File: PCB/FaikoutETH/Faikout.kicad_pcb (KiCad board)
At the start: 2 copper layers, 70 x 70 mm, 70 parts, among them J1 1x5, J2 TC2030-USB-NL, J3 Reset, J4 RJ45_LED, Q1 BSS138PS, U1 KSZ8851SNL, U4 ESP32-S3-MINI-1, U5 TPS62933, Y1 Crystal_GND24

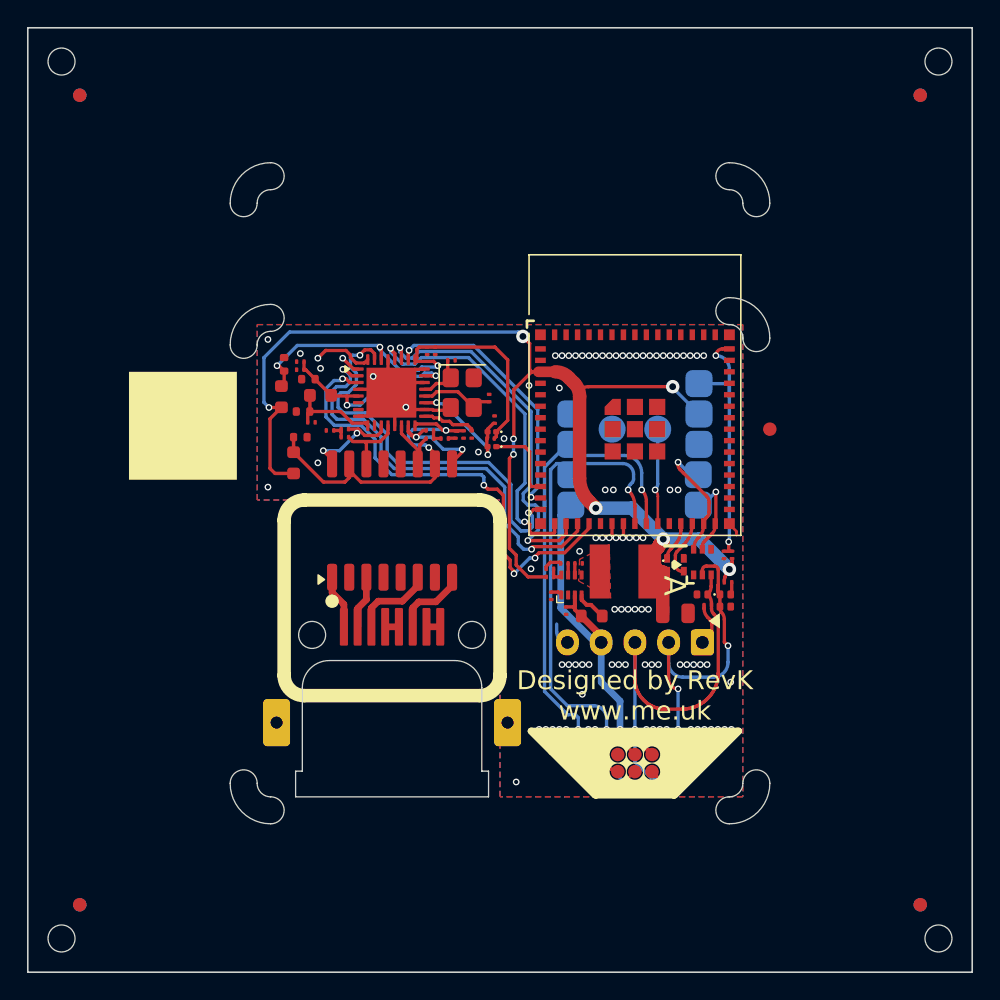
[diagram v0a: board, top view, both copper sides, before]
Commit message: Rotate
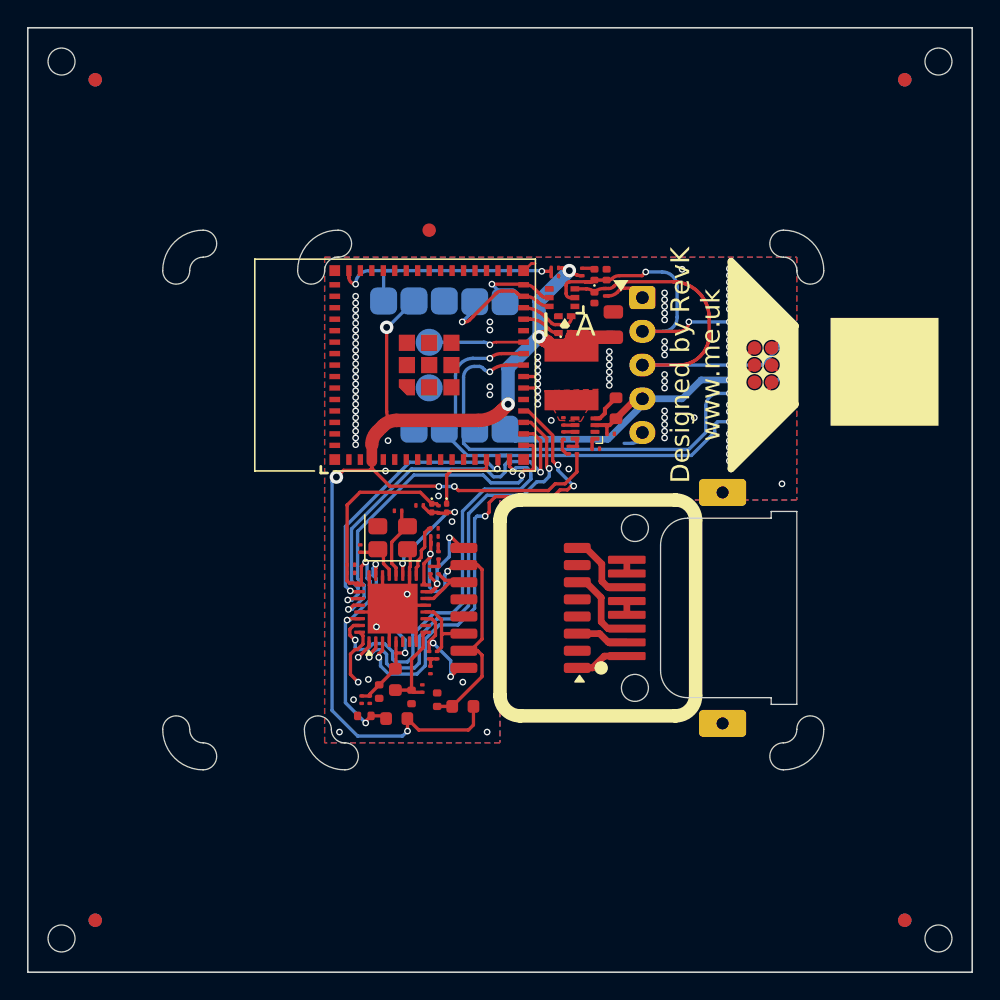
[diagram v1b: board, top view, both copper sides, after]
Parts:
- moved V5 32.5 mm to (112.0, 65.0), turned to 90 degrees
- moved V6 31.1 mm to (157.0, 65.0), turned to 90 degrees
- moved J2 31.0 mm to (154.5, 55.0), turned to -90 degrees
- moved FID2 29.2 mm to (129.8, 45.0), turned to 0 degrees
- moved C23 26.7 mm to (124.9, 81.0), turned to 180 degrees
- moved D3 26.1 mm to (142.9, 48.3), turned to -90 degrees
- moved J1 25.9 mm to (145.6, 50.0), turned to -90 degrees
- moved J4 25.9 mm to (151.5, 73.0), turned to 90 degrees
- moved D4 25.6 mm to (142.0, 48.3), turned to 90 degrees
- moved C9 25.5 mm to (124.7, 79.8), turned to -90 degrees
- moved V3 25.5 mm to (135.0, 47.0), turned to 0 degrees
- moved V4 25.5 mm to (135.0, 83.0), turned to 0 degrees
- moved R2 25.4 mm to (141.1, 48.1), turned to 90 degrees
- moved FB5 25.3 mm to (127.3, 81.2), turned to 0 degrees
- moved R3 25.0 mm to (139.1, 47.8), turned to 180 degrees
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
